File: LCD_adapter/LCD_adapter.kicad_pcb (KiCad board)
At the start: 2 copper layers, 24.8 x 52.1 mm, 3 parts, among them U1 RC1602A

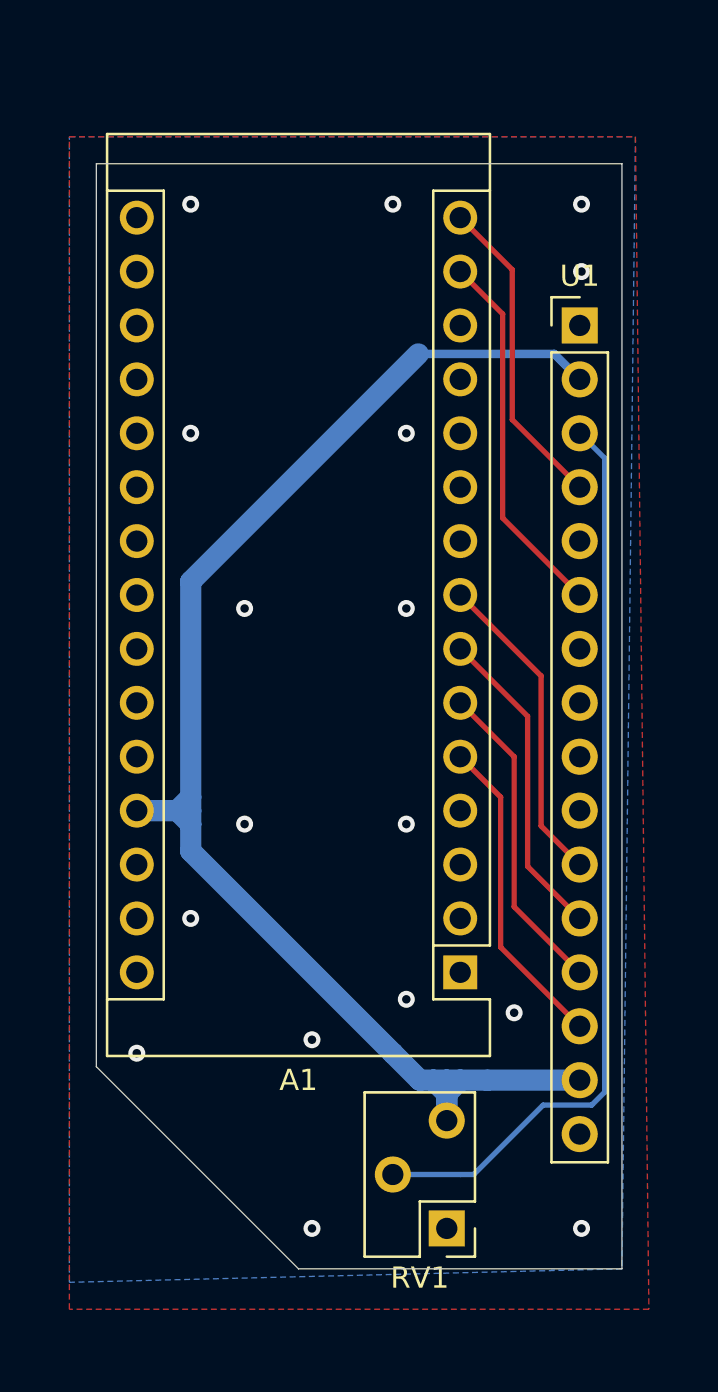
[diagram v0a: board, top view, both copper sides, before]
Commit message: version 1 complete
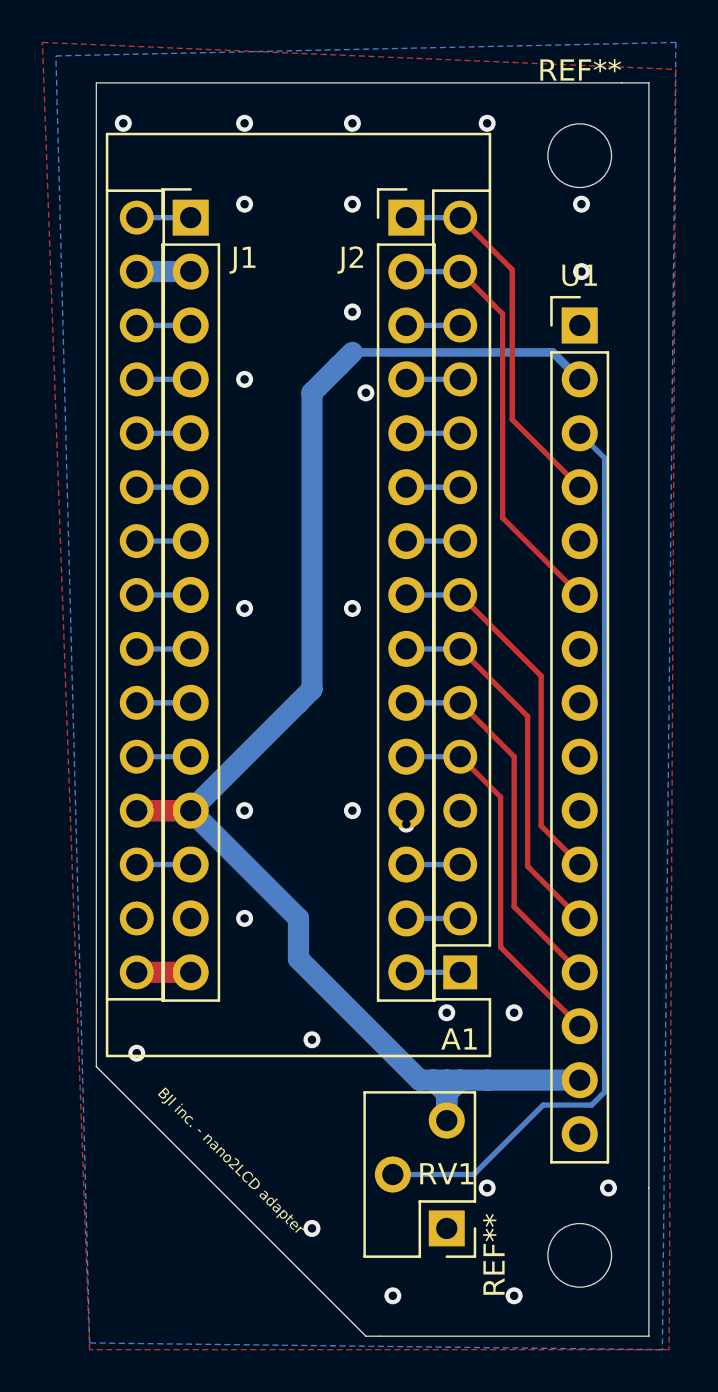
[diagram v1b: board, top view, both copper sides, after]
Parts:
- added J1: Conn_01x15_Male, Connector_PinHeader_2.54mm:PinHeader_1x15_P2.54mm_Vertical, F.Cu at (153.7, 64.8)
- added J2: Conn_01x15_Male, Connector_PinHeader_2.54mm:PinHeader_1x15_P2.54mm_Vertical, F.Cu at (163.8, 64.8)
- added REF**: MountingHole_3mm, MountingHole:MountingHole_3mm, F.Cu at (172.0, 61.9)
- added REF**: MountingHole_3mm, MountingHole:MountingHole_3mm, F.Cu at (172.0, 113.7)
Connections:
- A1 pad 1: Net-(A1-Pad1) -> /D1
- A1 pad 10: Net-(A1-Pad10) -> /D7
- A1 pad 11: Net-(A1-Pad11) -> /D8
- A1 pad 12: Net-(A1-Pad12) -> /D9
- A1 pad 13: Net-(A1-Pad13) -> /D10
- A1 pad 16: Net-(A1-Pad16) -> /D13
- A1 pad 17: Net-(A1-Pad17) -> /3V3
- A1 pad 18: Net-(A1-Pad18) -> /AREF
- A1 pad 19: Net-(A1-Pad19) -> /A0
- A1 pad 2: Net-(A1-Pad2) -> /D0
- A1 pad 20: Net-(A1-Pad20) -> /A1
- A1 pad 21: Net-(A1-Pad21) -> /A2
- A1 pad 22: Net-(A1-Pad22) -> /A3
- A1 pad 23: Net-(A1-Pad23) -> /A4
- A1 pad 24: Net-(A1-Pad24) -> /A5
- A1 pad 25: Net-(A1-Pad25) -> /A6
- A1 pad 26: Net-(A1-Pad26) -> /A7
- A1 pad 28: Net-(A1-Pad28) -> /nRST
- A1 pad 3: Net-(A1-Pad3) -> /nRST
- A1 pad 30: Net-(A1-Pad30) -> /Vin
- A1 pad 9: Net-(A1-Pad9) -> /D6
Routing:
- net /nRST: track 0.00 -> 5.08 mm
- net VDD: track 68.1 -> 70.7 mm
- net /D3: track 15.0 -> 17.6 mm
- net /D2: track 15.0 -> 17.6 mm
- net /D12: track 15.0 -> 17.6 mm
- net /Vin: track 0.00 -> 2.54 mm
- net /D9: track 0.00 -> 2.54 mm
- net /D8: track 0.00 -> 2.54 mm, vias 0 -> 1
- net /D7: track 0.00 -> 2.54 mm
- net /D6: track 0.00 -> 2.54 mm
- net /D4: track 15.0 -> 17.6 mm
- net /D13: track 0.00 -> 2.54 mm
- net /D11: track 17.6 -> 20.1 mm
- net /D10: track 0.00 -> 2.54 mm
- net /D1: track 0.00 -> 2.54 mm
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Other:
- board size 24.8 x 52.1 mm -> 26 x 59.1 mm
- board text added: "3V3"
- board text added: "5V"
- board text added: "A0"
- board text added: "A1"
- board text added: "A2"
- board text added: "A3"
- board text added: "A4"
- board text added: "A5"
- board text added: "A6"
- board text added: "A7"
- board text added: "BJI inc. - nano2LCD adapter"
- board text added: "D10"
- board text added: "D11"
- board text added: "D12"
- board text added: "D13"
- board text added: "D2"
- board text added: "D3"
- board text added: "D4"
- board text added: "D5"
- board text added: "D6"
- board text added: "D7"
- board text added: "D8"
- board text added: "D9"
- board text added: "GND"
- board text added: "REF"
- board text added: "RST"
- board text added: "RXD"
- board text added: "TXD"
- board text added: "VIN"
